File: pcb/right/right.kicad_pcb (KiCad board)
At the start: 2 copper layers, 31.8 x 72.4 mm, 21 parts, among them J1 Conn_01x07

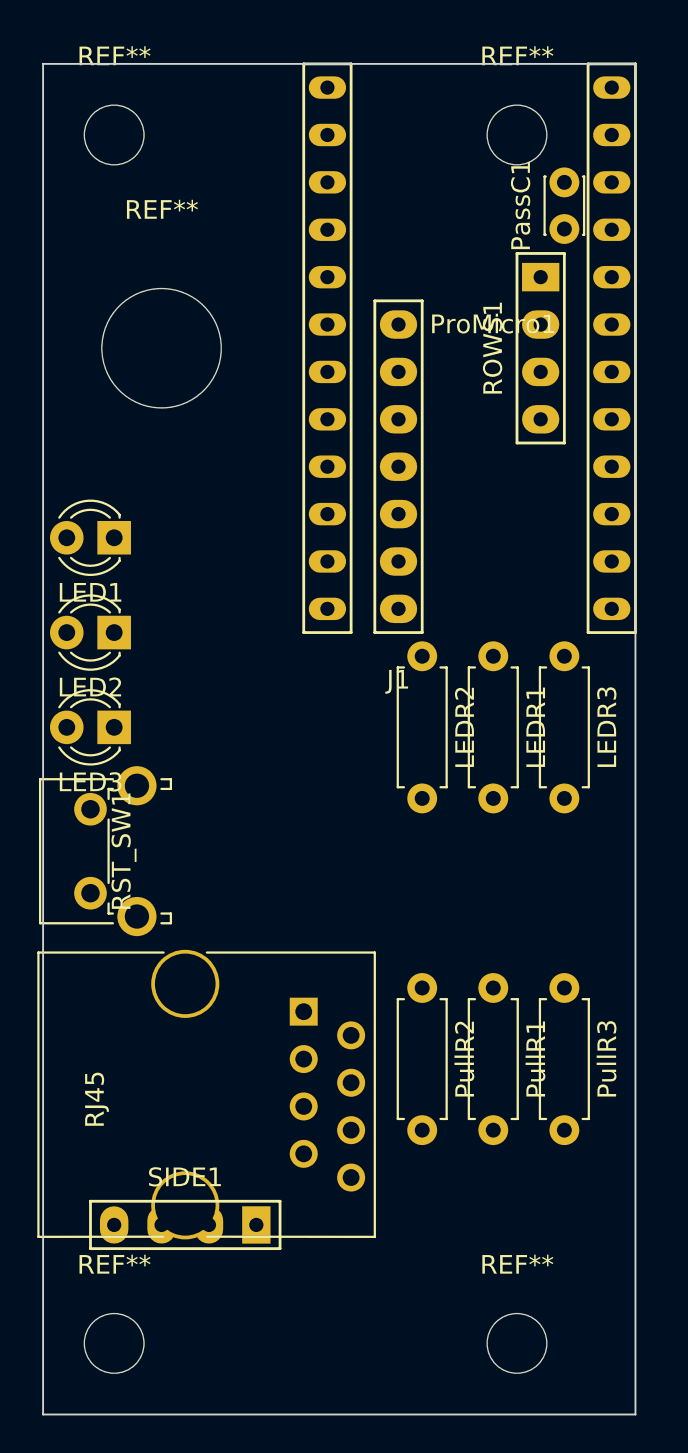
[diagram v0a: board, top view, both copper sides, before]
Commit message: improve pcb size
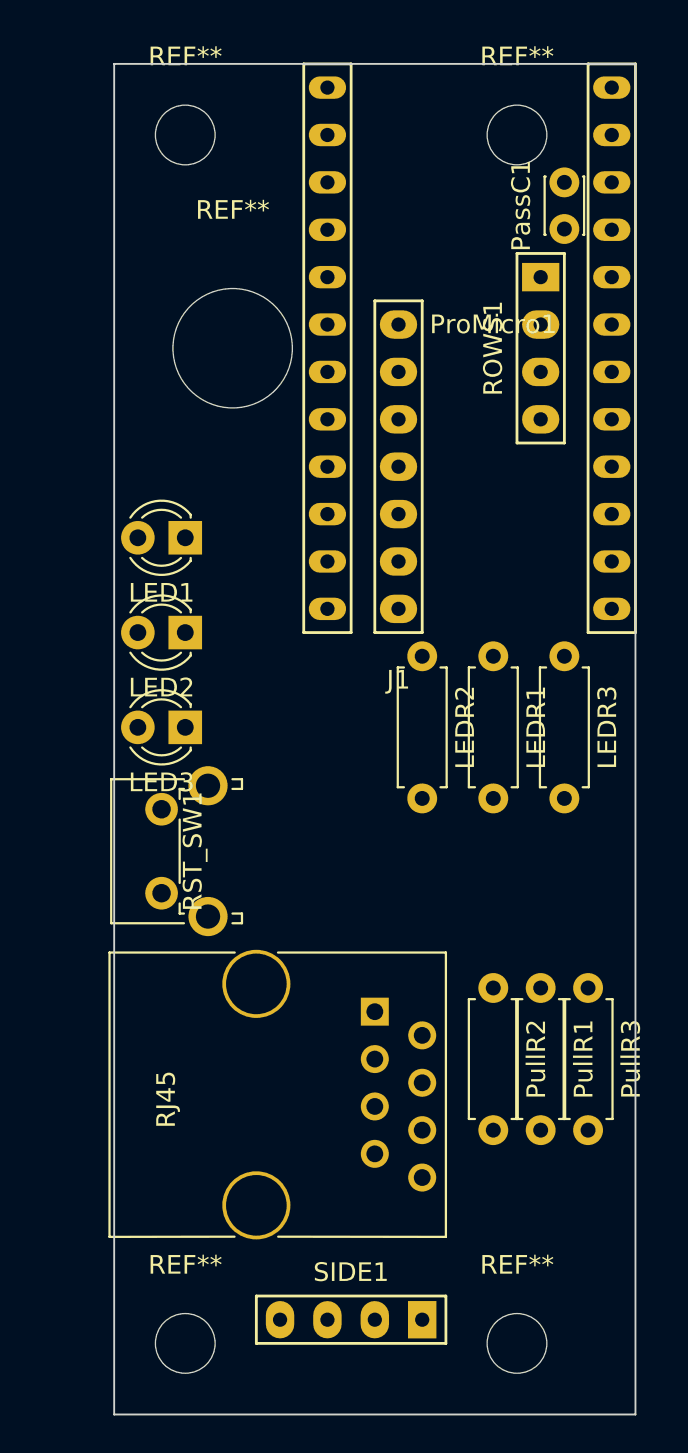
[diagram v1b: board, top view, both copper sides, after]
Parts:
- moved SIDE1 10.2 mm to (48.3, 96.5)
- moved PullR2 3.81 mm to (55.9, 78.7)
- moved RJ45 3.81 mm to (49.5, 80.0)
- moved RST_SW1 3.81 mm to (38.1, 73.7)
- moved LED1 3.81 mm to (39.4, 54.6)
- moved LED2 3.81 mm to (39.4, 59.7)
- moved LED3 3.81 mm to (39.4, 64.8)
- moved REF** 3.81 mm to (41.9, 44.5)
- moved REF** 3.81 mm to (39.4, 33.0)
- moved REF** 3.81 mm to (39.4, 97.8)
- moved PullR1 2.54 mm to (58.4, 78.7)
- moved PullR3 1.27 mm to (61.0, 78.7)
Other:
- board size 31.8 x 72.4 mm -> 27.9 x 72.4 mm
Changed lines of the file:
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@@
     (links 44)
     (no_connects 44)
-    (area 28.539857 27.842 66.710143 103.068)
+    (area 29.809857 27.842 66.710143 103.068)
     (thickness 1.6)
     (drawings 4)
@@
   )
   (module LEDs:LED_D3.0mm (layer F.Cu)
-    (at 35.56 54.61 180)
+    (at 39.37 54.61 180)
     (descr "LED, diameter 3.0mm, 2 pins")
     (tags "LED diameter 3.0mm 2 pins")
@@
   )
   (module LEDs:LED_D3.0mm (layer F.Cu)
-    (at 35.56 59.69 180)
+    (at 39.37 59.69 180)
     (descr "LED, diameter 3.0mm, 2 pins")
     (tags "LED diameter 3.0mm 2 pins")
@@
   )
   (module LEDs:LED_D3.0mm (layer F.Cu)
-    (at 35.56 64.77 180)
+    (at 39.37 64.77 180)
     (descr "LED, diameter 3.0mm, 2 pins")
     (tags "LED diameter 3.0mm 2 pins")
@@
   )
   (module Resistors_THT:R_Axial_DIN0207_L6.3mm_D2.5mm_P7.62mm_Horizontal (layer F.Cu)
-    (at 55.88 78.74 270)
+    (at 58.42 78.74 270)
     (descr "Resistor, Axial_DIN0207 series, Axial, Horizontal, pin pitch=7.62mm, 0.25W = 1/4W, length*diameter=6.3*2.5mm^2, http://cdn-reichelt.de/documents/datenblatt/B400/1_4W%23YAG.pdf")
     (tags "Resistor Axial_DIN0207 series Axial Horizontal pin pitch 7.62mm 0.25W = 1/4W length 6.3mm diameter 2.5mm")
@@
   )
   (module Resistors_THT:R_Axial_DIN0207_L6.3mm_D2.5mm_P7.62mm_Horizontal (layer F.Cu)
-    (at 52.07 78.74 270)
+    (at 55.88 78.74 270)
     (descr "Resistor, Axial_DIN0207 series, Axial, Horizontal, pin pitch=7.62mm, 0.25W = 1/4W, length*diameter=6.3*2.5mm^2, http://cdn-reichelt.de/documents/datenblatt/B400/1_4W%23YAG.pdf")
     (tags "Resistor Axial_DIN0207 series Axial Horizontal pin pitch 7.62mm 0.25W = 1/4W length 6.3mm diameter 2.5mm")
@@
   )
   (module Resistors_THT:R_Axial_DIN0207_L6.3mm_D2.5mm_P7.62mm_Horizontal (layer F.Cu)
-    (at 59.69 78.74 270)
+    (at 60.96 78.74 270)
     (descr "Resistor, Axial_DIN0207 series, Axial, Horizontal, pin pitch=7.62mm, 0.25W = 1/4W, length*diameter=6.3*2.5mm^2, http://cdn-reichelt.de/documents/datenblatt/B400/1_4W%23YAG.pdf")
     (tags "Resistor Axial_DIN0207 series Axial Horizontal pin pitch 7.62mm 0.25W = 1/4W length 6.3mm diameter 2.5mm")
@@
   )
   (module Connectors:RJ45_8 (layer F.Cu)
-    (at 45.72 80.01 270)
+    (at 49.53 80.01 270)
     (tags RJ45)
     (fp_text reference RJ45 (at 4.7 11.18 270) (layer F.SilkS)
@@
   )
   (module Buttons_Switches_THT:SW_Tactile_SPST_Angled_PTS645Vx31-2LFS (layer F.Cu)
-    (at 34.29 73.66 90)
+    (at 38.1 73.66 90)
     (descr "tactile switch SPST right angle, PTS645VL31-2 LFS")
     (tags "tactile switch SPST angled PTS645VL31-2 LFS C&K Button")
@@
   )
   (module 4x6t2:Wirepad_01x04 (layer F.Cu)
-    (at 39.37 91.44 270)
+    (at 48.26 96.52 270)
     (fp_text reference SIDE1 (at -2.54 0 360) (layer F.SilkS)
       (effects (font (size 1 1) (thickness 0.15)))
@@
   )
   (module Mounting_Holes:MountingHole_6.4mm_M6 (layer F.Cu)
-    (at 38.1 44.45)
+    (at 41.91 44.45)
     (descr "Mounting Hole 6.4mm, no annular, M6")
     (tags "mounting hole 6.4mm no annular m6")
@@
   )
   (module Mounting_Holes:MountingHole_3.2mm_M3 (layer F.Cu)
-    (at 35.56 33.02)
+    (at 39.37 33.02)
     (descr "Mounting Hole 3.2mm, no annular, M3")
     (tags "mounting hole 3.2mm no annular m3")
@@
   )
   (module Mounting_Holes:MountingHole_3.2mm_M3 (layer F.Cu)
-    (at 35.56 97.79)
+    (at 39.37 97.79)
     (descr "Mounting Hole 3.2mm, no annular, M3")
     (tags "mounting hole 3.2mm no annular m3")
@@
       (net 6 /COL5))
   )
-  (gr_line (start 31.75 101.6) (end 63.5 101.6) (layer Edge.Cuts) (width 0.1))
+  (gr_line (start 35.56 101.6) (end 63.5 101.6) (layer Edge.Cuts) (width 0.1))
   (gr_line (start 63.5 29.21) (end 63.5 101.6) (layer Edge.Cuts) (width 0.1))
-  (gr_line (start 31.75 29.21) (end 31.75 101.6) (layer Edge.Cuts) (width 0.1))
-  (gr_line (start 63.5 29.21) (end 31.75 29.21) (layer Edge.Cuts) (width 0.1))
+  (gr_line (start 35.56 29.21) (end 35.56 101.6) (layer Edge.Cuts) (width 0.1))
+  (gr_line (start 63.5 29.21) (end 35.56 29.21) (layer Edge.Cuts) (width 0.1))
 )
